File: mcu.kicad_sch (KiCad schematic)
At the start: 8 parts, among them J10 LOLIN-S3 (R), J11 ESP32-S3-DEVKITC-1 (L), J12 ESP32-S3-DEVKITC-1 (R), J13 LOLIN-S2-MINI (L Outer), J14 LOLIN-S2-MINI (R Outer), J15 LOLIN-S2-MINI (L Inner), J16 LOLIN-S2-MINI (R Inner), J9 LOLIN-S3 (L)

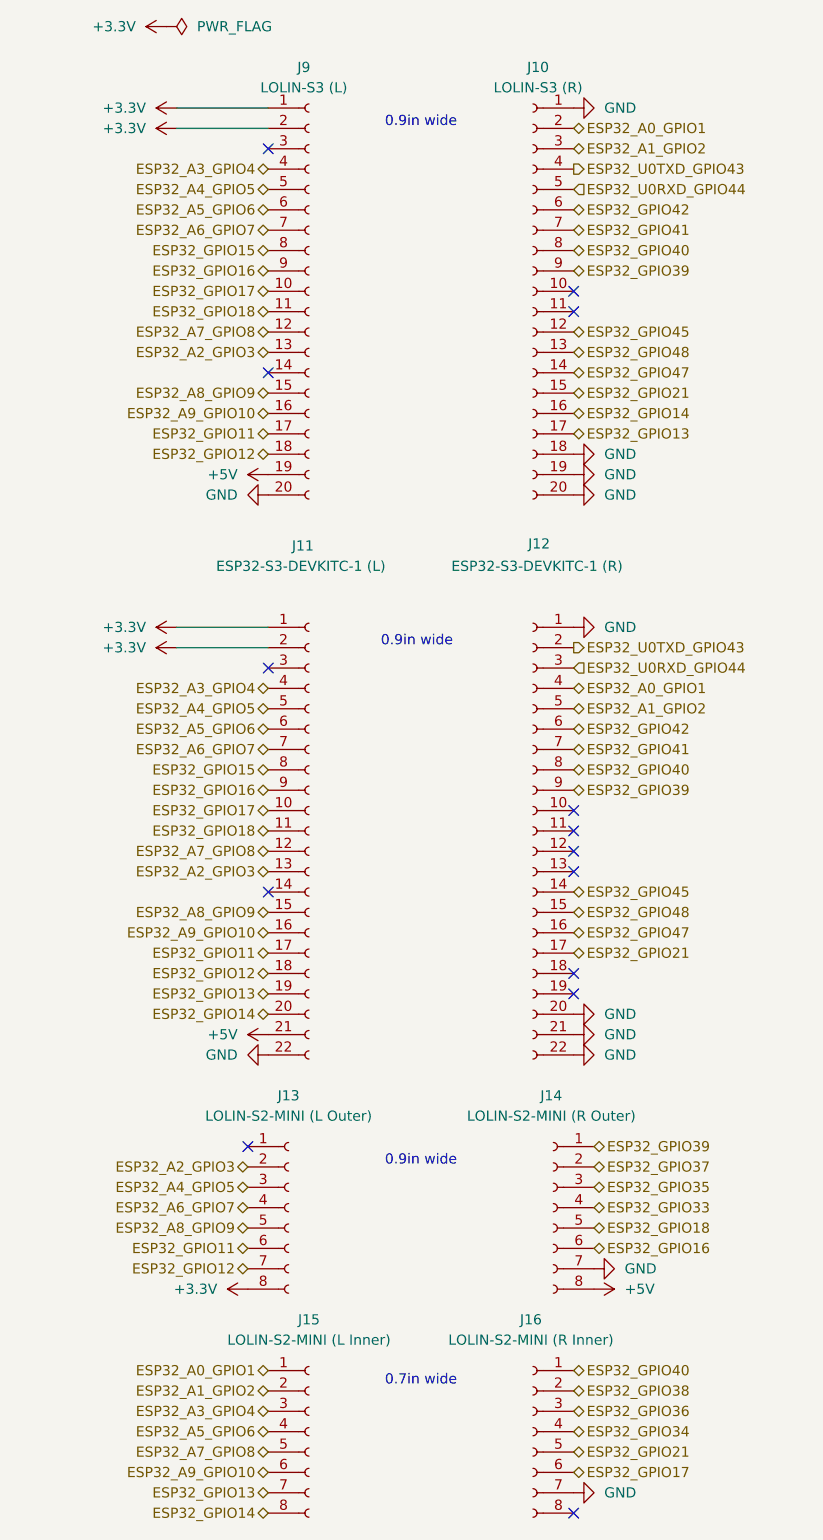
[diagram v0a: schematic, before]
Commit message: Place all components
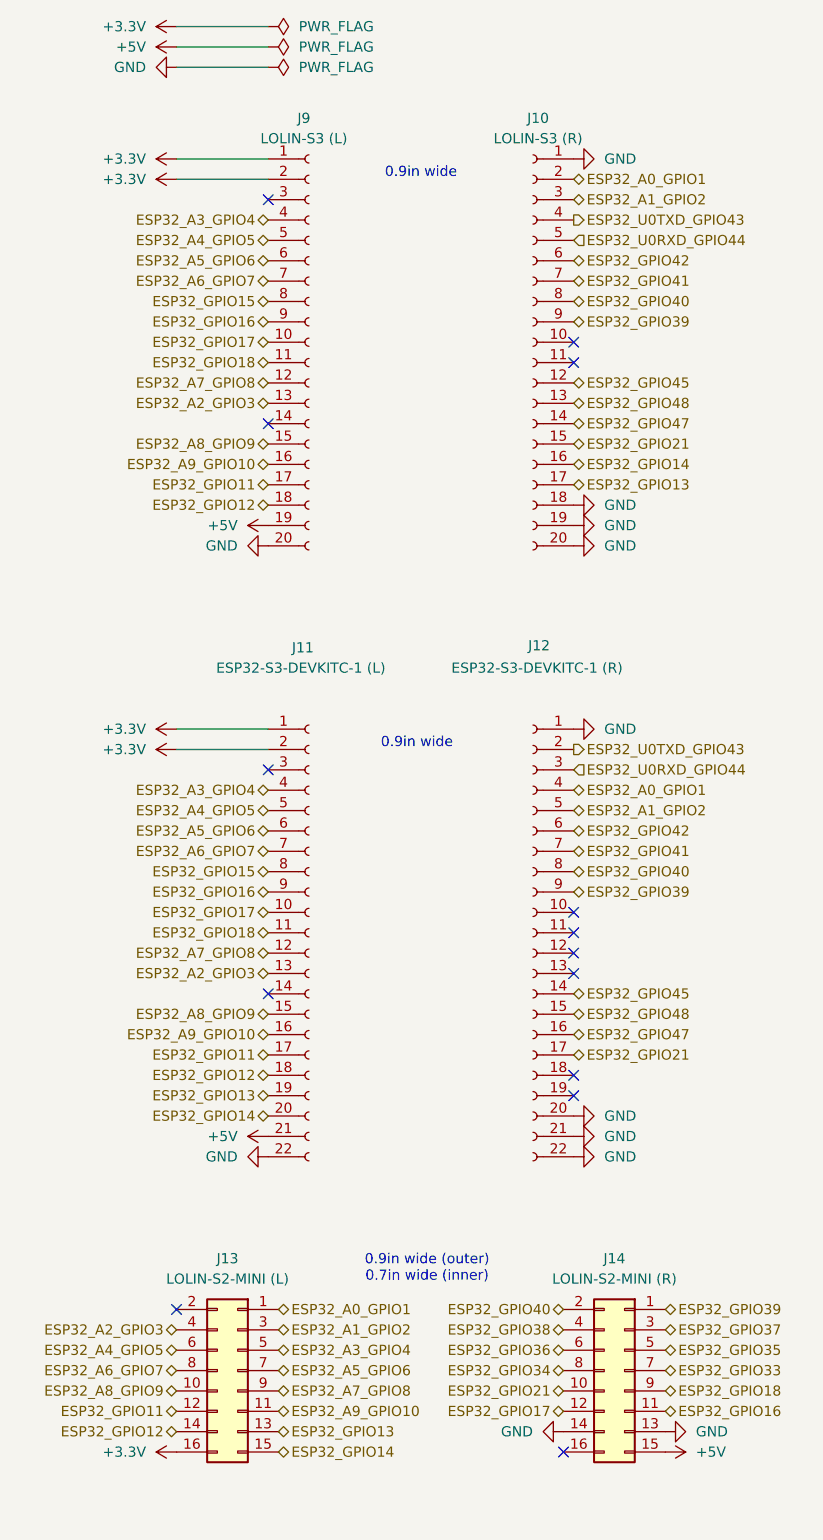
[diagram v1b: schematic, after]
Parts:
- removed J13: LOLIN-S2-MINI (L Outer), Connector_PinHeader_2.54mm:PinHeader_1x08_P2.54mm_Vertical, symbol Connector:Conn_01x08_Socket
- removed J14: LOLIN-S2-MINI (R Outer), Connector_PinHeader_2.54mm:PinHeader_1x08_P2.54mm_Vertical, symbol Connector:Conn_01x08_Socket
- removed J15: LOLIN-S2-MINI (L Inner), Connector_PinHeader_2.54mm:PinHeader_1x08_P2.54mm_Vertical, symbol Connector:Conn_01x08_Socket
- removed J16: LOLIN-S2-MINI (R Inner), Connector_PinHeader_2.54mm:PinHeader_1x08_P2.54mm_Vertical, symbol Connector:Conn_01x08_Socket
- added J13: LOLIN-S2-MINI (L), Connector_PinSocket_2.54mm:PinSocket_2x08_P2.54mm_Vertical, symbol Connector_Generic:Conn_02x08_Odd_Even
- added J14: LOLIN-S2-MINI (R), Connector_PinSocket_2.54mm:PinSocket_2x08_P2.54mm_Vertical, symbol Connector_Generic:Conn_02x08_Odd_Even
- J11, J12: footprint Connector_PinHeader_2.54mm:PinHeader_1x22_P2.54mm_Vertical -> Connector_PinSocket_2.54mm:PinSocket_1x22_P2.54mm_Vertical
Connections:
- net +3.3V: now also J13.16 (Pin_16)
- net +5V: now also J14.15 (Pin_15)
- net ESP32_A0_GPIO1: now also J13.1 (Pin_1)
- net ESP32_A1_GPIO2: now also J13.3 (Pin_3)
- net ESP32_A2_GPIO3: now also J13.4 (Pin_4)
- net ESP32_A3_GPIO4: now also J13.5 (Pin_5)
- net ESP32_A4_GPIO5: now also J13.6 (Pin_6)
- net ESP32_A5_GPIO6: now also J13.7 (Pin_7)
- net ESP32_A6_GPIO7: now also J13.8 (Pin_8)
- net ESP32_A7_GPIO8: now also J13.9 (Pin_9)
- net ESP32_A8_GPIO9: now also J13.10 (Pin_10)
- net ESP32_A9_GPIO10: now also J13.11 (Pin_11)
- net ESP32_GPIO11: now also J13.12 (Pin_12)
- net ESP32_GPIO12: now also J13.14 (Pin_14)
- net ESP32_GPIO13: now also J13.13 (Pin_13)
- net ESP32_GPIO14: now also J13.15 (Pin_15)
- net ESP32_GPIO16: now also J14.11 (Pin_11)
- net ESP32_GPIO17: now also J14.12 (Pin_12)
- net ESP32_GPIO18: now also J14.9 (Pin_9)
- net ESP32_GPIO21: now also J14.10 (Pin_10)
- net ESP32_GPIO33: now also J14.7 (Pin_7)
- net ESP32_GPIO34: now also J14.8 (Pin_8)
- net ESP32_GPIO35: now also J14.5 (Pin_5)
- net ESP32_GPIO36: now also J14.6 (Pin_6)
- net ESP32_GPIO37: now also J14.3 (Pin_3)
- net ESP32_GPIO38: now also J14.4 (Pin_4)
- net ESP32_GPIO39: now also J14.1 (Pin_1)
- net ESP32_GPIO40: now also J14.2 (Pin_2)
- net GND: now also J14.13 (Pin_13), J14.14 (Pin_14)
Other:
- note added: "0.9in wide (outer) 0.7in wide (inner)"
- note removed: "0.7in wide"
- moved on the sheet: J10, J11, J12, J9
